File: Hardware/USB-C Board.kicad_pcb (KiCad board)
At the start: 2 copper layers, 34 x 34 mm, 52 parts, among them J1 USB_C_Receptacle_USB2.0, J2 Conn_01x04_Male, J3 Conn_01x02_Male, J4 Conn_01x02_Male, J5 Conn_01x02_Male, J6 Conn_01x02_Male, J9 QWIIC_Stackable, Q1 DMP3013SFV, SW1 SW_Push, U1 AMS1117-3.3, U3 STUSB4500QTR

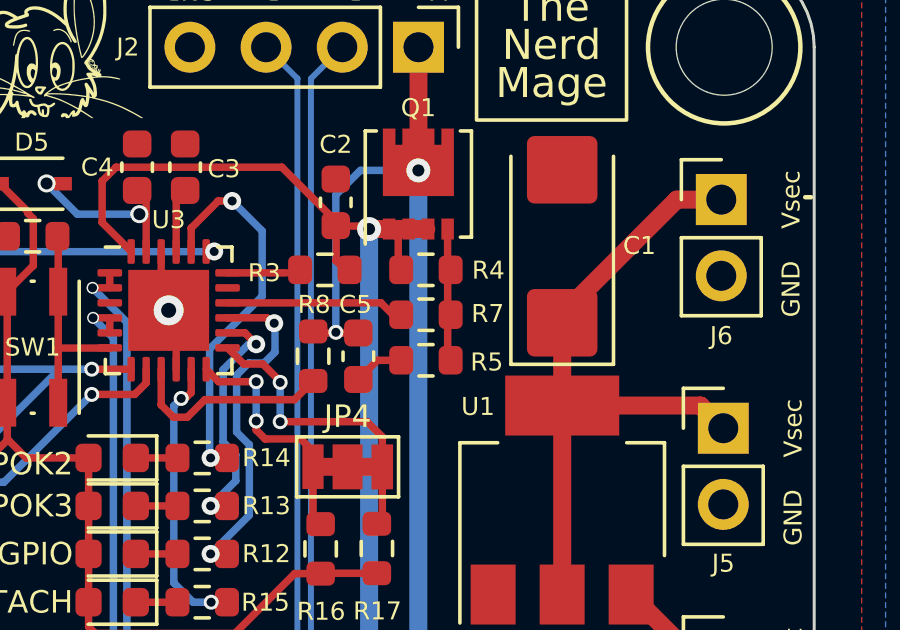
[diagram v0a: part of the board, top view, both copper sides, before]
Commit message: fiddlin' with stuff...
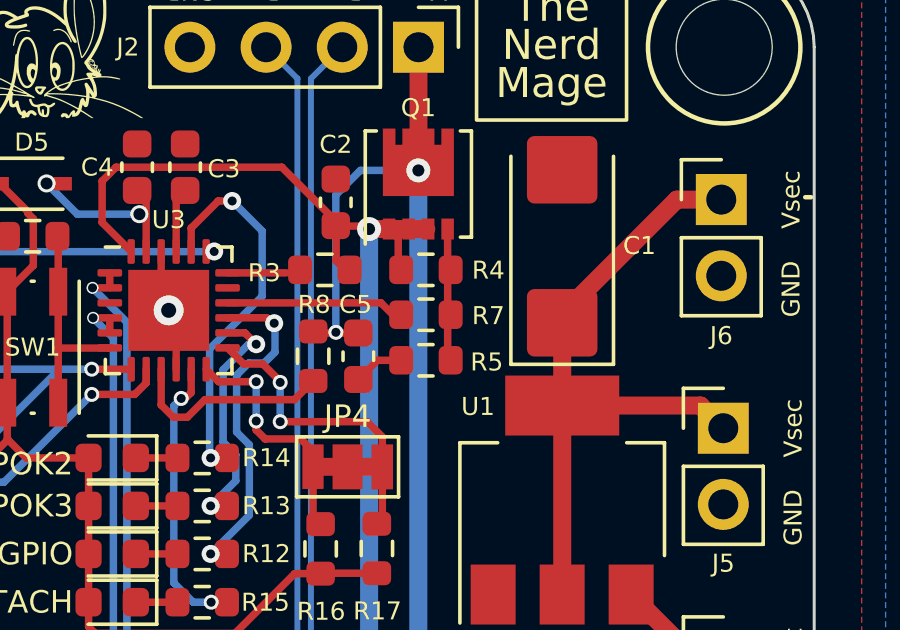
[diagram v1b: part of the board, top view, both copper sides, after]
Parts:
- turned R7 to 180 degrees
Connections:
- R7 pad 1: Net-(R7-Pad1) -> Net-(Q1-Pad4)
- R7 pad 2: Net-(Q1-Pad4) -> Net-(U3-Pad16)
- U3 pad 16: Net-(R7-Pad1) -> Net-(U3-Pad16)
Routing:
- net Net-(U3-Pad16): track 0.00 -> 5.96 mm
- net Net-(R7-Pad1): track 5.96 -> 0.00 mm
